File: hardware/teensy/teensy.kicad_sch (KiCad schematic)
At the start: 99 parts, among them J4 CONN_083.5MM-8, J5 CONN_083.5MM-8, J6 CONN_083.5MM-8, J7 CONN_083.5MM-8, J8 CONN_023.5MM, J9 CONN_023.5MM, U1 Teensy3.5

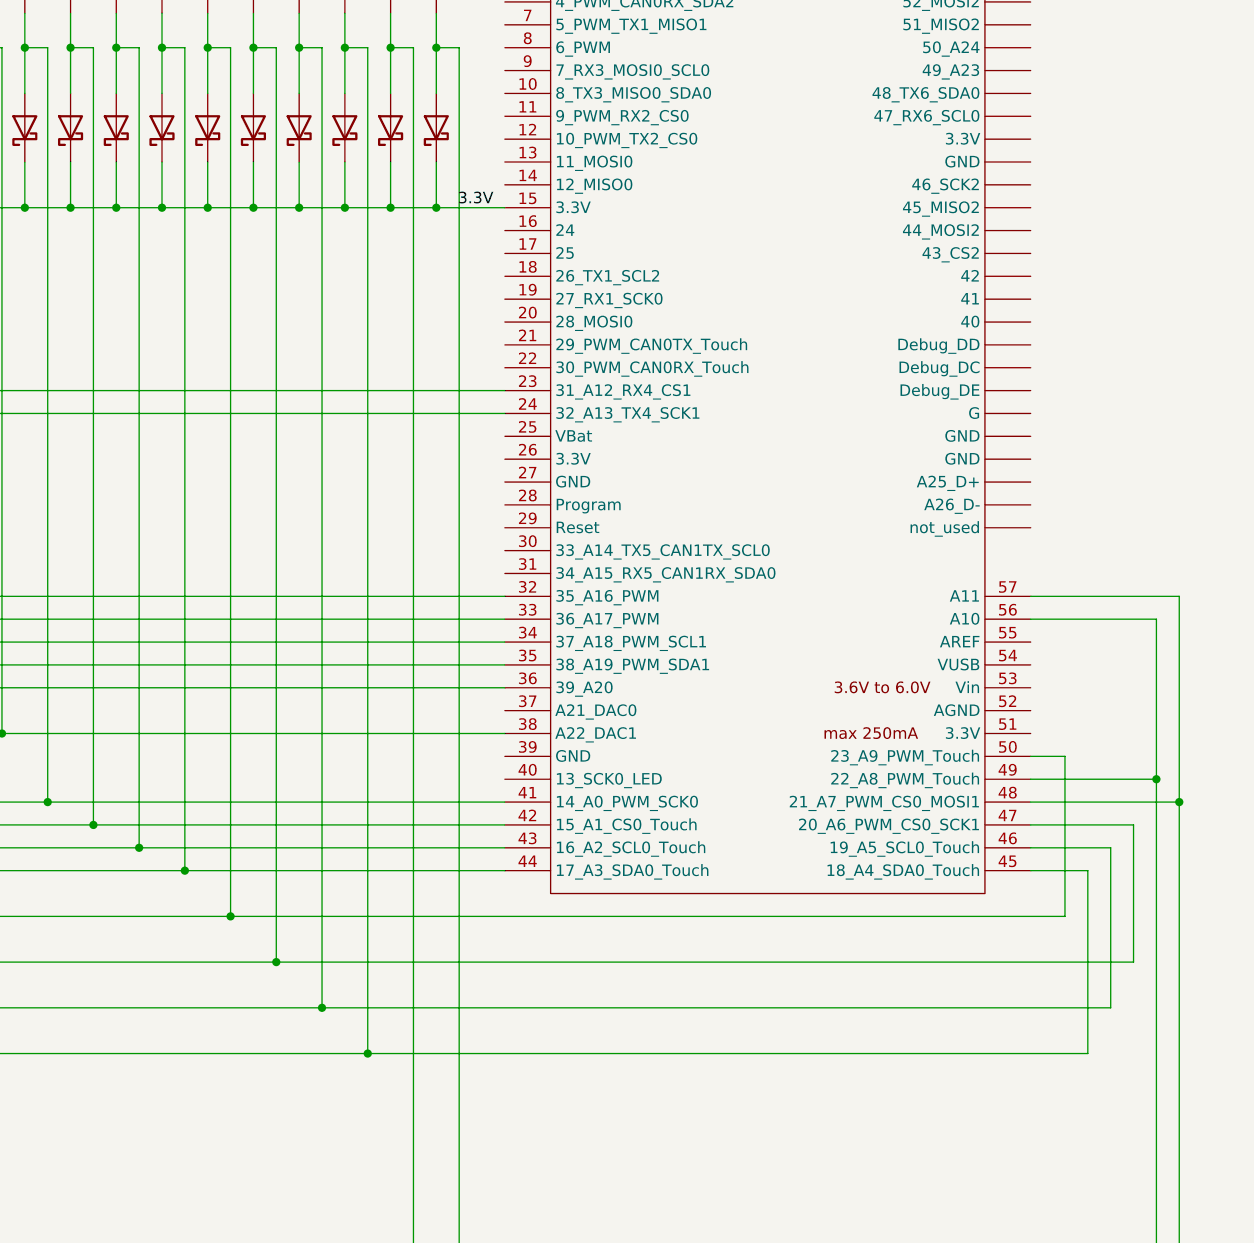
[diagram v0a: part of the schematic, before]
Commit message: prettier traces, removed smt thing
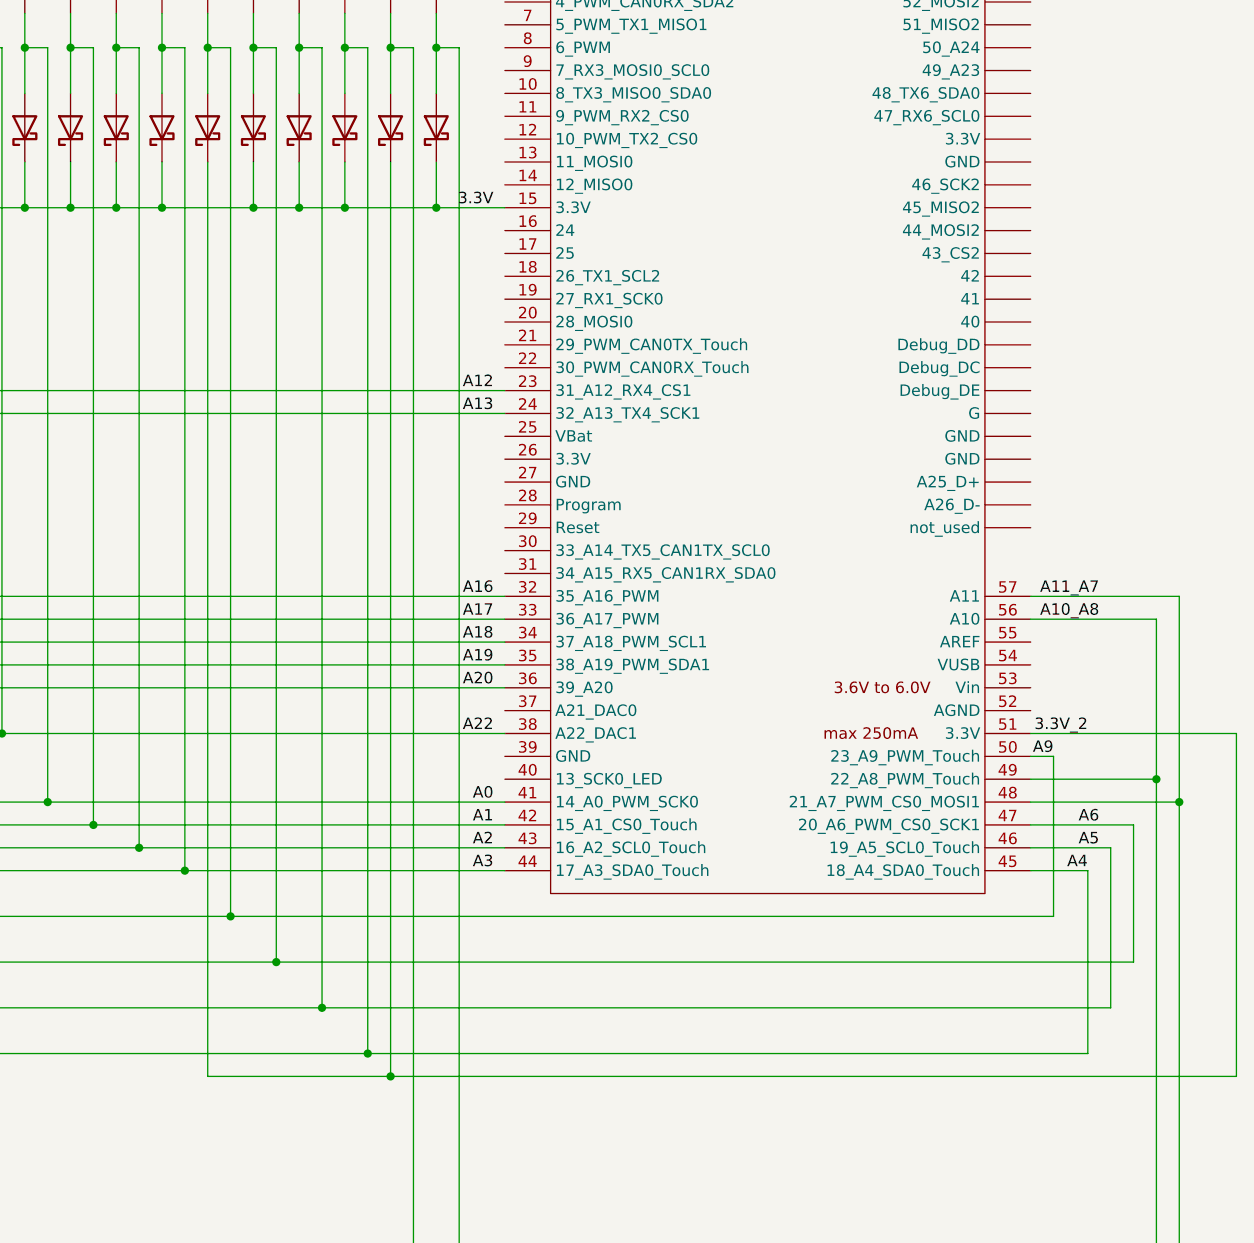
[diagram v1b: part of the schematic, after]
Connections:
- net 3.3V: no longer D26.1 (K), D34.1 (K)
- net A9: now reaches D25.1 (K), D26.2 (A), R35.P$2 (2), U1.50 (23_A9_PWM_Touch)
- net A13: now reaches D3.1 (K), D4.2 (A), R24.P$2 (2), U1.24 (32_A13_TX4_SCK1)
- net A18: now reaches D10.2 (A), D9.1 (K), R27.P$2 (2), U1.34 (37_A18_PWM_SCL1)
- net A1: now reaches D19.1 (K), D20.2 (A), R32.P$2 (2), U1.42 (15_A1_CS0_Touch)
- net A6: now reaches D27.1 (K), D28.2 (A), R36.P$2 (2), U1.47 (20_A6_PWM_CS0_SCK1)
- net A4: now reaches D31.1 (K), D32.2 (A), R38.P$2 (2), U1.45 (18_A4_SDA0_Touch)
- net A22: now reaches D15.1 (K), D16.2 (A), R30.P$2 (2), U1.38 (A22_DAC1)
- net A5: now reaches D29.1 (K), D30.2 (A), R37.P$2 (2), U1.46 (19_A5_SCL0_Touch)
- net A2: now reaches D21.1 (K), D22.2 (A), R33.P$2 (2), U1.43 (16_A2_SCL0_Touch)
- net A16: now reaches D5.1 (K), D6.2 (A), R25.P$2 (2), U1.32 (35_A16_PWM)
- net A19: now reaches D11.1 (K), D12.2 (A), R28.P$2 (2), U1.35 (38_A19_PWM_SDA1)
- net A3: now reaches D23.1 (K), D24.2 (A), R34.P$2 (2), U1.44 (17_A3_SDA0_Touch)
- net A20: now reaches D13.1 (K), D14.2 (A), R29.P$2 (2), U1.36 (39_A20)
- net A12: now reaches D1.1 (K), D2.2 (A), R23.P$2 (2), U1.23 (31_A12_RX4_CS1)
- net A17: now reaches D7.1 (K), D8.2 (A), R26.P$2 (2), U1.33 (36_A17_PWM)
- net A0: now reaches D17.1 (K), D18.2 (A), R31.P$2 (2), U1.41 (14_A0_PWM_SCK0)
- net 3.3V_2: now reaches U1.51 (3.3V)
- net 3.3V_2: now also D26.1 (K), D34.1 (K)
- net L1_SCALED renamed A11_A7
- net L2_SCALED renamed A10_A8
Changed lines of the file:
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@@
   (junction (at 274.32 120.65) (diameter 0) (color 0 0 0 0))
   (junction (at 274.32 138.43) (diameter 0) (color 0 0 0 0))
-  (junction (at 274.32 156.21) (diameter 0) (color 0 0 0 0))
   (junction (at 276.86 234.95) (diameter 0) (color 0 0 0 0))
   (junction (at 279.4 120.65) (diameter 0) (color 0 0 0 0))
@@
   (junction (at 294.64 120.65) (diameter 0) (color 0 0 0 0))
   (junction (at 294.64 138.43) (diameter 0) (color 0 0 0 0))
-  (junction (at 294.64 156.21) (diameter 0) (color 0 0 0 0))
+  (junction (at 294.64 252.73) (diameter 0) (color 0 0 0 0))
   (junction (at 297.18 284.48) (diameter 0) (color 0 0 0 0))
   (junction (at 299.72 120.65) (diameter 0) (color 0 0 0 0))
@@
     (stroke (width 0) (type solid) (color 0 0 0 0))
   )
-  (wire (pts (xy 269.24 156.21) (xy 274.32 156.21))
+  (wire (pts (xy 269.24 156.21) (xy 279.4 156.21))
     (stroke (width 0) (type solid) (color 0 0 0 0))
   )
@@
     (stroke (width 0) (type solid) (color 0 0 0 0))
   )
-  (wire (pts (xy 274.32 151.13) (xy 274.32 156.21))
+  (wire (pts (xy 274.32 151.13) (xy 274.32 252.73))
     (stroke (width 0) (type solid) (color 0 0 0 0))
   )
-  (wire (pts (xy 274.32 156.21) (xy 279.4 156.21))
+  (wire (pts (xy 274.32 252.73) (xy 294.64 252.73))
     (stroke (width 0) (type solid) (color 0 0 0 0))
   )
@@
     (stroke (width 0) (type solid) (color 0 0 0 0))
   )
-  (wire (pts (xy 276.86 234.95) (xy 369.57 234.95))
+  (wire (pts (xy 276.86 234.95) (xy 368.3 234.95))
     (stroke (width 0) (type solid) (color 0 0 0 0))
   )
@@
     (stroke (width 0) (type solid) (color 0 0 0 0))
   )
-  (wire (pts (xy 289.56 156.21) (xy 294.64 156.21))
+  (wire (pts (xy 289.56 156.21) (xy 299.72 156.21))
     (stroke (width 0) (type solid) (color 0 0 0 0))
   )
@@
     (stroke (width 0) (type solid) (color 0 0 0 0))
   )
-  (wire (pts (xy 294.64 151.13) (xy 294.64 156.21))
+  (wire (pts (xy 294.64 252.73) (xy 294.64 151.13))
     (stroke (width 0) (type solid) (color 0 0 0 0))
   )
-  (wire (pts (xy 294.64 156.21) (xy 299.72 156.21))
+  (wire (pts (xy 294.64 252.73) (xy 388.62 252.73))
     (stroke (width 0) (type solid) (color 0 0 0 0))
   )
@@
     (stroke (width 0) (type solid) (color 0 0 0 0))
   )
-  (wire (pts (xy 365.76 217.17) (xy 369.57 217.17))
+  (wire (pts (xy 365.76 214.63) (xy 388.62 214.63))
+    (stroke (width 0) (type solid) (color 0 0 0 0))
+  )
+  (wire (pts (xy 365.76 217.17) (xy 368.3 217.17))
     (stroke (width 0) (type solid) (color 0 0 0 0))
   )
@@
     (stroke (width 0) (type solid) (color 0 0 0 0))
   )
-  (wire (pts (xy 369.57 217.17) (xy 369.57 234.95))
+  (wire (pts (xy 368.3 217.17) (xy 368.3 234.95))
     (stroke (width 0) (type solid) (color 0 0 0 0))
   )
@@
     (stroke (width 0) (type solid) (color 0 0 0 0))
   )
+  (wire (pts (xy 388.62 214.63) (xy 388.62 252.73))
+    (stroke (width 0) (type solid) (color 0 0 0 0))
+  )
   (label "L2" (at 83.82 284.48 180)
     (effects (font (size 1.27 1.27)) (justify right bottom))
@@
     (effects (font (size 1.27 1.27)) (justify right bottom))
   )
+  (label "A12" (at 306.07 176.53 180)
+    (effects (font (size 1.27 1.27)) (justify right bottom))
+  )
+  (label "A13" (at 306.07 179.07 180)
+    (effects (font (size 1.27 1.27)) (justify right bottom))
+  )
+  (label "A16" (at 306.07 199.39 180)
+    (effects (font (size 1.27 1.27)) (justify right bottom))
+  )
+  (label "A17" (at 306.07 201.93 180)
+    (effects (font (size 1.27 1.27)) (justify right bottom))
+  )
+  (label "A18" (at 306.07 204.47 180)
+    (effects (font (size 1.27 1.27)) (justify right bottom))
+  )
+  (label "A19" (at 306.07 207.01 180)
+    (effects (font (size 1.27 1.27)) (justify right bottom))
+  )
+  (label "A20" (at 306.07 209.55 180)
+    (effects (font (size 1.27 1.27)) (justify right bottom))
+  )
+  (label "A22" (at 306.07 214.63 180)
+    (effects (font (size 1.27 1.27)) (justify right bottom))
+  )
+  (label "A0" (at 306.07 222.25 180)
+    (effects (font (size 1.27 1.27)) (justify right bottom))
+  )
+  (label "A1" (at 306.07 224.79 180)
+    (effects (font (size 1.27 1.27)) (justify right bottom))
+  )
+  (label "A2" (at 306.07 227.33 180)
+    (effects (font (size 1.27 1.27)) (justify right bottom))
+  )
+  (label "A3" (at 306.07 229.87 180)
+    (effects (font (size 1.27 1.27)) (justify right bottom))
+  )
+  (label "A9" (at 368.3 217.17 180)
+    (effects (font (size 1.27 1.27)) (justify right bottom))
+  )
+  (label "3.3V_2" (at 372.11 214.63 180)
+    (effects (font (size 1.27 1.27)) (justify right bottom))
+  )
+  (label "A4" (at 372.11 229.87 180)
+    (effects (font (size 1.27 1.27)) (justify right bottom))
+  )
+  (label "A11_A7" (at 373.38 199.39 180)
+    (effects (font (size 1.27 1.27)) (justify right bottom))
+  )
+  (label "A10_A8" (at 373.38 201.93 180)
+    (effects (font (size 1.27 1.27)) (justify right bottom))
+  )
+  (label "A6" (at 373.38 224.79 180)
+    (effects (font (size 1.27 1.27)) (justify right bottom))
+  )
+  (label "A5" (at 373.38 227.33 180)
+    (effects (font (size 1.27 1.27)) (justify right bottom))
+  )
   (symbol (lib_id "SparkFun-Resistors:RESISTORAXIAL-0.3") (at 118.11 176.53 0) (unit 1)
     (in_bom yes) (on_board yes)
@@
       (effects (font (size 1.27 1.27)) hide)
     )
-    (property "Footprint" "teensy:Teensy35_36" (id 2) (at 336.55 175.26 0)
+    (property "Footprint" "teensy:Teensy35_36_EMON" (id 2) (at 336.55 175.26 0)
       (effects (font (size 1.27 1.27)) hide)
     )
